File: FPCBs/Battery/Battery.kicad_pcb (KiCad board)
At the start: 2 copper layers, 20.5 x 23 mm, 6 parts

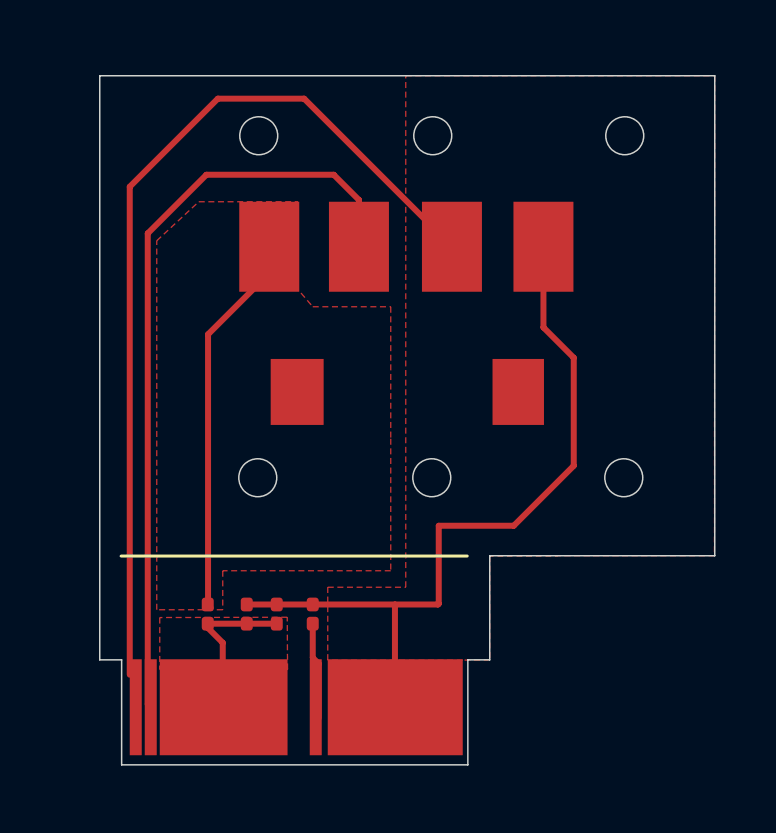
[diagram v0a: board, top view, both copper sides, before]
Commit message: Battery fpcb
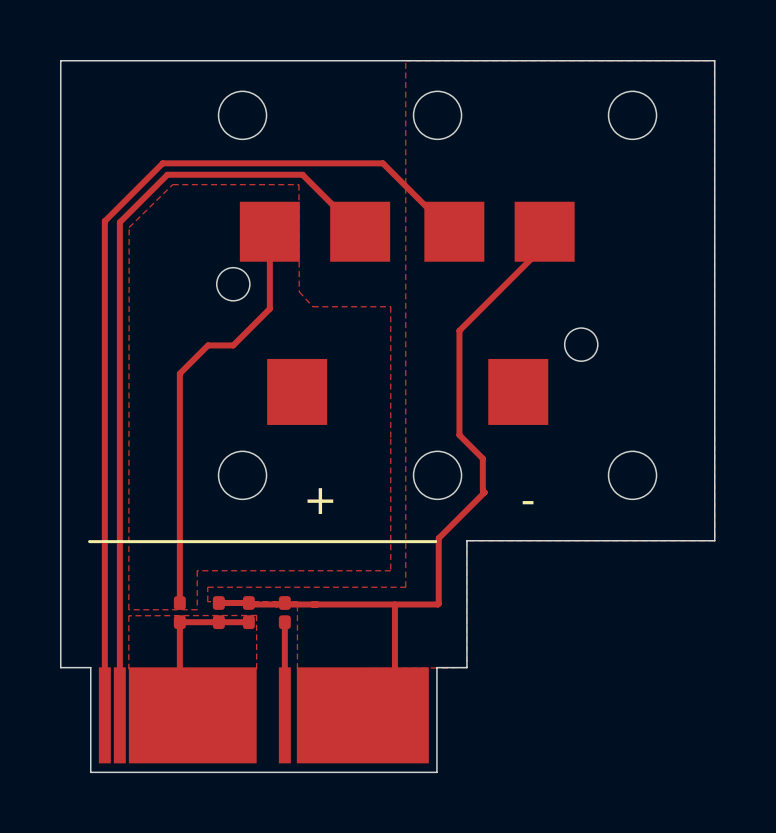
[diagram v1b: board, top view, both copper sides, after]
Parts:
- moved Power_Connector_Camera1 1.06 mm to (139.7, 91.7)
- moved F1 0.93 mm to (137.0, 88.1)
- moved R1 0.93 mm to (140.5, 88.1)
- moved C1 0.93 mm to (138.3, 88.1)
- moved C2 0.93 mm to (139.3, 88.1)
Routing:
- net Net-(Power_Connector_Battery1-+): track 12.5 -> 14.1 mm
- net Net-(Power_Connector_Battery1--): track 26.3 -> 25.4 mm
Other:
- board size 20.5 x 23 mm -> 21.8 x 23.7 mm
- board text added: "+"
- board text added: "-"
